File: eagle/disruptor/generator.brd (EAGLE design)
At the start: 76.2 x 120.7 mm, 29 parts, among them IC1 NE555, IC2 74ALS04N, IC3 IR2110, IC4 7805TV, J1 PIN2F061.100, J2 PIN2F061.100, J3 PIN2F061.100, J4 PIN2F061.100, J5 PIN2F061.100, J6 PIN2F061.100, Q1 STP11NM60, Q2 STP11NM60

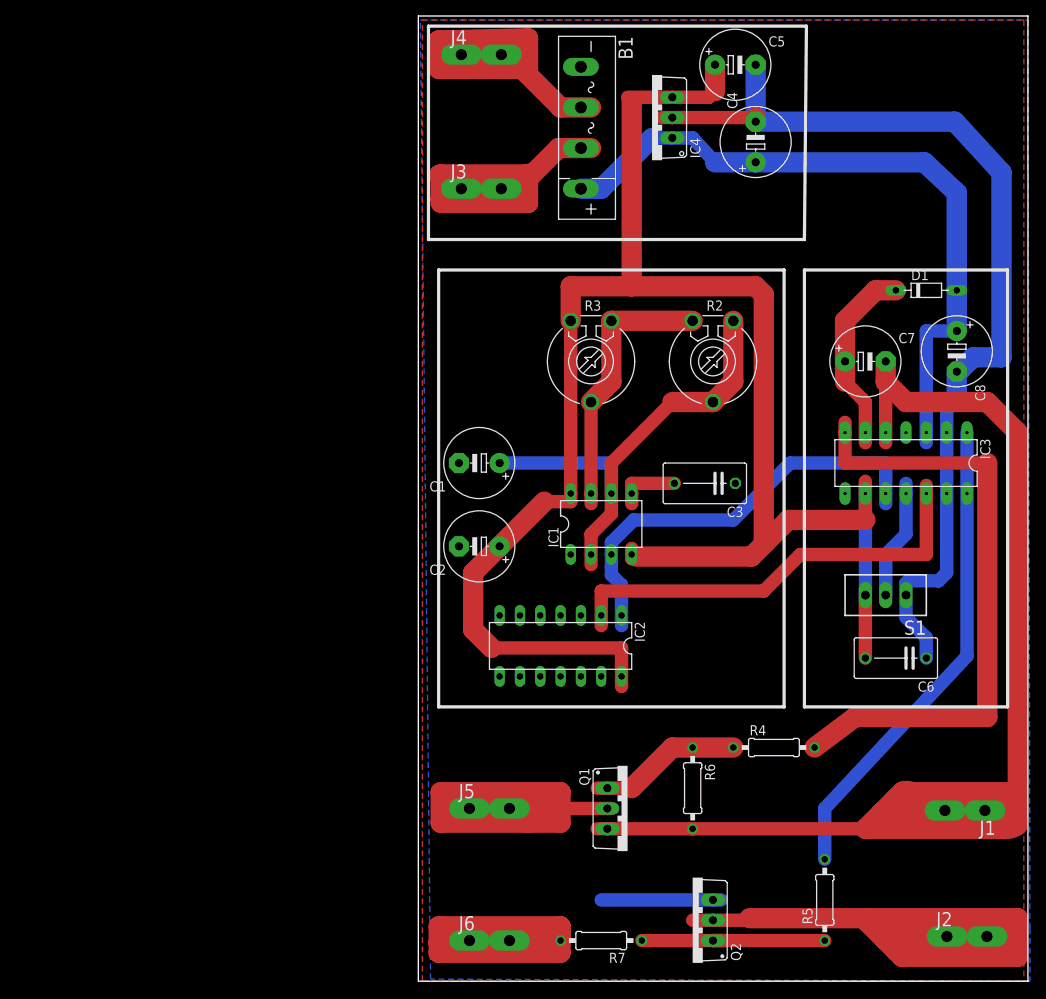
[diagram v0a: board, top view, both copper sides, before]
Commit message: pre-round 2
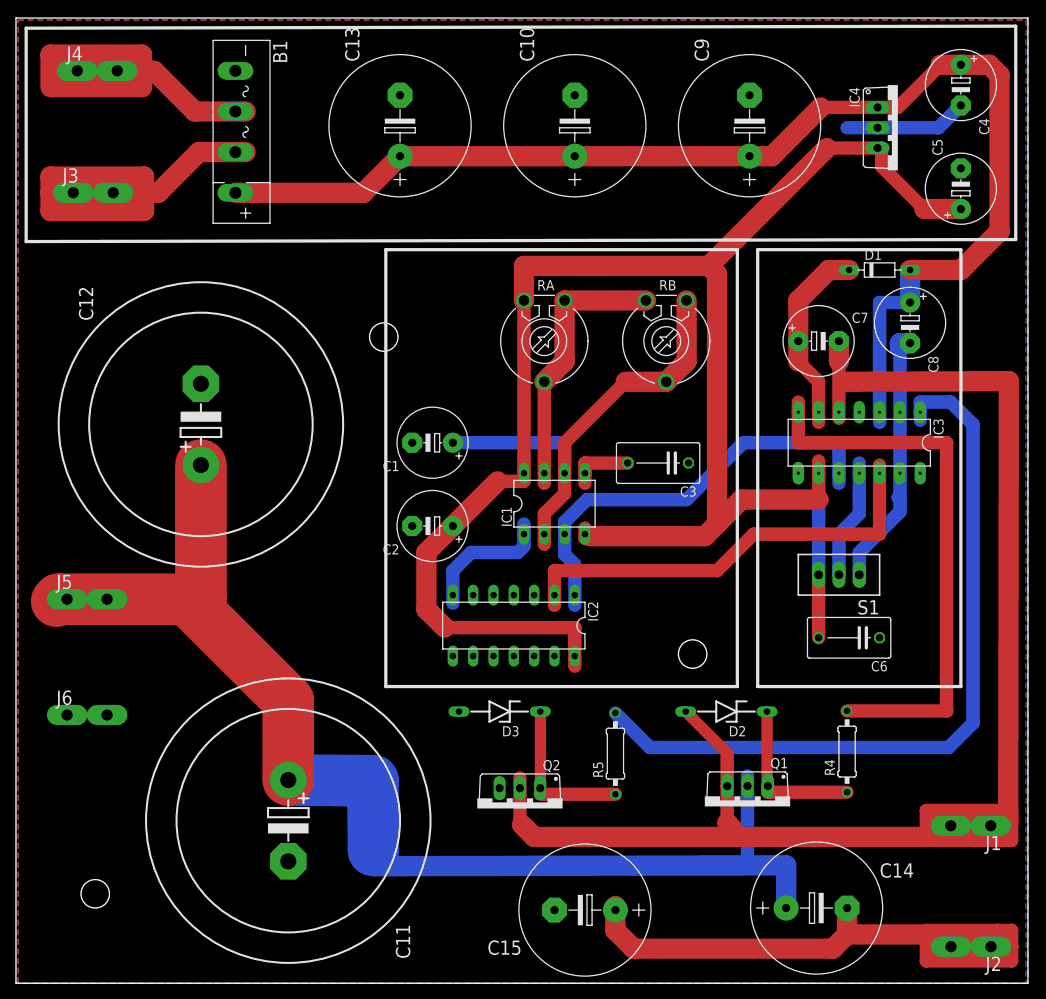
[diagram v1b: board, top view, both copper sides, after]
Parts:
- removed R2, R3: (no value), pot:LI10
- removed R6, R7: 1M, rcl:0207/10
- added C10, C13, C9: (no value), resistor:E7,5-18
- added C11, C12: 2200, resistor:EB35D
- added C14, C15: 560u, rcl:E7,5-16
- added D2, D3: (no value), diode:ZDIO-10
- added RA, RB: 10k, pot:LI10
- C1: value .1u -> .01u
- C7: value 1u -> min 12 nF
- R4, R5: value 100 -> 10
- moved J6 57.7 mm to (-41.4, 33.3)
- moved J5 56.7 mm to (-41.4, 47.8)
- moved J3 48.5 mm to (-40.6, 98.6)
- moved J4 48.0 mm to (-40.1, 113.8)
- moved B1 43.2 mm to (-22.9, 106.2)
- moved C5 32.2 mm to (67.8, 99.1), turned to 90 degrees
- moved R5 31.9 mm to (24.6, 28.4)
- moved IC4 30.8 mm to (59.9, 106.7), turned to 270 degrees
- moved C4 26.6 mm to (67.8, 112.0), turned to 270 degrees
- moved Q2 25.7 mm to (12.7, 21.6), turned to 180 degrees
- moved Q1 15.0 mm to (41.1, 21.8), turned to 180 degrees
- moved R4 9.16 mm to (53.6, 28.7), turned to 90 degrees
- moved C8 6.84 mm to (61.5, 82.3)
- moved C7 6.37 mm to (50.0, 80.0)
- moved C1 6.37 mm to (1.78, 67.3)
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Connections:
- removed net N$13: J5.A1, J5.A2, Q1.D
- removed net TRANS1: C7.-, IC3.5, J1.A1, J1.A2, Q1.S, R6.2
- removed net TRANS2: J2.A1, J2.A2, Q2.D
- new net N$6: C11.+, C12.+, C14.+, J5.A1, J5.A2, Q1.D
- new net N$8: C14.-, C15.+, J2.A1, J2.A2
- new net TRANS: C7.-, D2.A, IC3.5, J1.A1, J1.A2, Q1.S, Q2.D
- net GND: now also C10.-, C11.-, C12.-, C13.-, C15.-, C9.-, D3.A; no longer R7.2
- net N$11: now also D3.C; no longer R7.1
- net N$12: now also D2.C; no longer R6.1
- net N$2: now also RB.A, RB.S; no longer R2.A, R2.S
- net N$7: now also RA.A, RA.S, RB.E; no longer R2.E, R3.A, R3.S
- net VCC: now also RA.E; no longer R3.E
- net VDD: now also C10.+, C13.+, C9.+
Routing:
- net TRANS: track 0.00 -> 223.5 mm
- net TRANS1: track 201.4 -> 0.00 mm
- net N$6: track 0.00 -> 149.6 mm
- net GND: track 190.0 -> 65.7 mm
- net TRANS2: track 114.5 -> 0.00 mm
- net N$8: track 0.00 -> 99.3 mm
- net VDD: track 87.5 -> 158.3 mm
- net N$13: track 62.5 -> 0.00 mm
- net LO: track 60.3 -> 95.1 mm
- net N$10: track 54.8 -> 63.5 mm
- net HO: track 77.5 -> 69.6 mm
- net N$11: track 24.1 -> 18.9 mm
- net VCC: track 228.9 -> 233.4 mm
- net N$12: track 19.1 -> 20.1 mm
- net N$9: track 60.0 -> 59.0 mm
- added copper zone on layer 1, net GND
- removed copper zone on layer 1, net N$4
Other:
- board size 76.2 x 120.7 mm -> 126.5 x 120.7 mm
